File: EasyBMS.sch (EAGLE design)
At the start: 143 parts, among them Q10 BSS84LT1G, Q11 BSS84LT1G, Q12 BSS84LT1G, Q13 BSS84LT1G, Q2 BSS84LT1G, Q3 BSS84LT1G, Q4 BSS84LT1G, Q5 BSS84LT1G, Q6 BSS84LT1G, Q7 BSS84LT1G, Q8 BSS84LT1G, Q9 BSS84LT1G

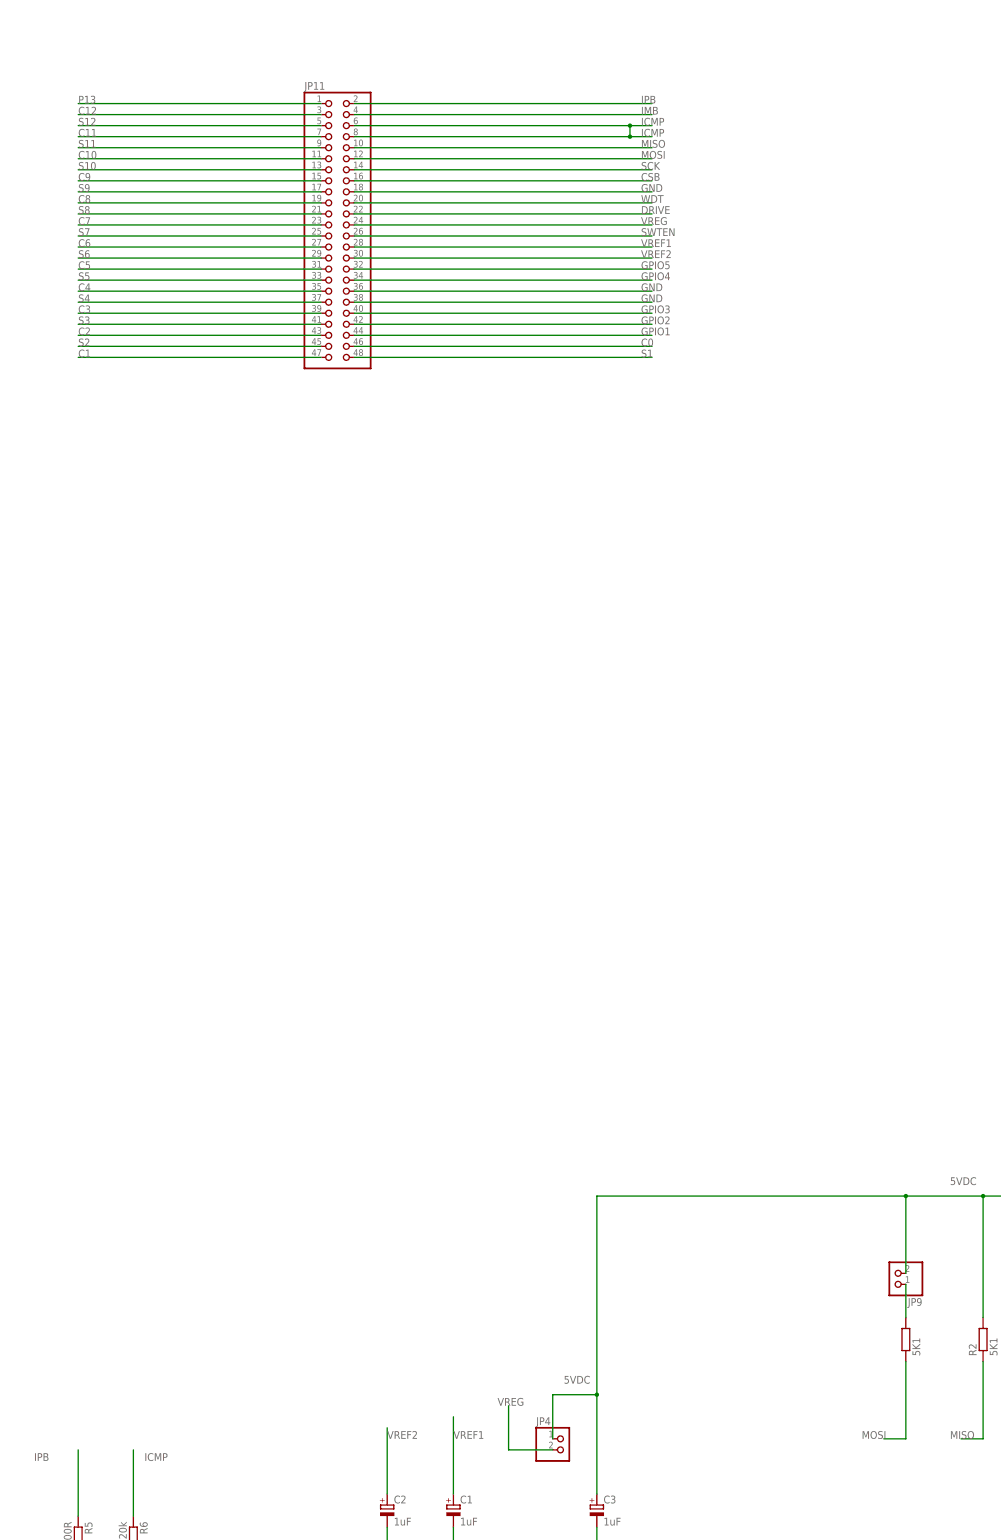
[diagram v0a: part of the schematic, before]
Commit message: new 2x20 header used
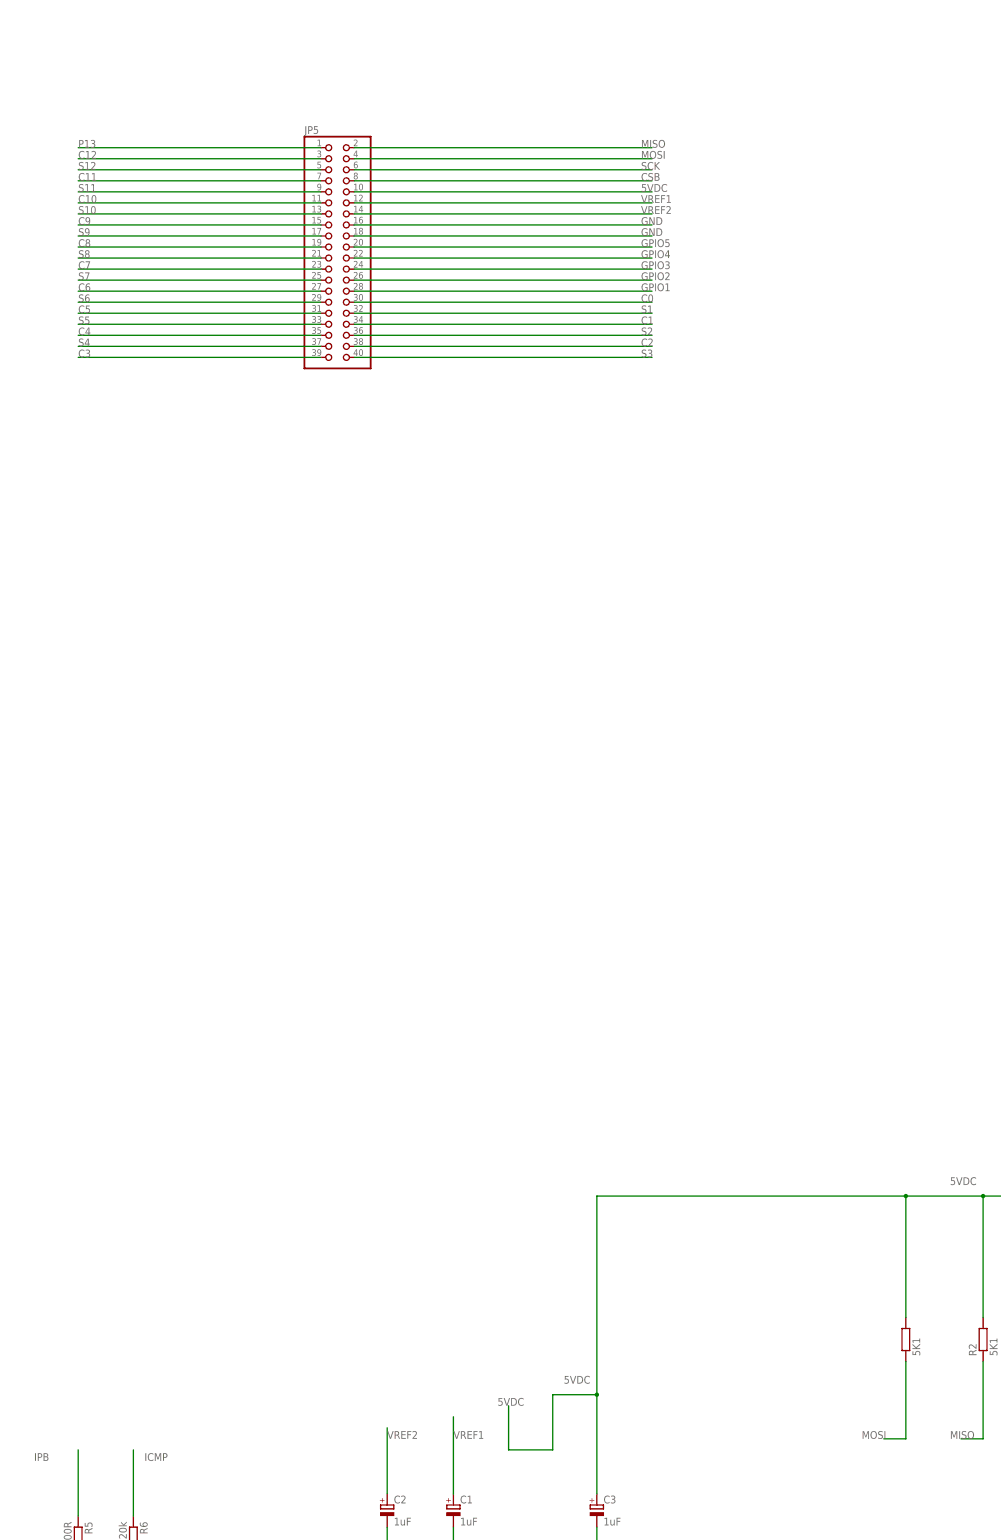
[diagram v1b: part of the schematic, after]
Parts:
- removed JP11: (no value), pinhead_own:PINHD-2X24
- removed JP4, JP9: (no value), pinhead_own:PINHD-1X2
- added JP5: (no value), pinhead:PINHD-2X20
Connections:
- removed net DRIVE: JP11.22
- removed net N$117: JP9.1, R1.2
- removed net SWTEN: JP11.26
- removed net VREG: JP11.24, JP4.2
- removed net WDT: JP11.20
- net 5VDC: now also JP5.10, R1.2; no longer JP4.1, JP9.2
- net C0: now also JP5.30; no longer JP11.46
- net C1: now also JP5.34; no longer JP11.47
- net C10: now also JP5.11; no longer JP11.11
- net C11: now also JP5.7; no longer JP11.7
- net C12: now also JP5.3; no longer JP11.3
- net C2: now also JP5.38; no longer JP11.43
- net C3: now also JP5.39; no longer JP11.39
- net C4: now also JP5.35; no longer JP11.35
- net C5: now also JP5.31; no longer JP11.31
- net C6: now also JP5.27; no longer JP11.27
- net C7: now also JP5.23; no longer JP11.23
- net C8: now also JP5.19; no longer JP11.19
- net C9: now also JP5.15; no longer JP11.15
- net CSB: now also JP5.8; no longer JP11.16
- net GND: now also JP5.16, JP5.18; no longer JP11.18, JP11.36, JP11.38
- net GPIO1: now also JP5.28; no longer JP11.44
- net GPIO2: now also JP5.26; no longer JP11.42
- net GPIO3: now also JP5.24; no longer JP11.40
- net GPIO4: now also JP5.22; no longer JP11.34
- net GPIO5: now also JP5.20; no longer JP11.32
- net ICMP: no longer JP11.6, JP11.8
- net IMB: no longer JP11.4
- net IPB: no longer JP11.2
- net MISO: now also JP5.2; no longer JP11.10
- net MOSI: now also JP5.4; no longer JP11.12
- net P13: now also JP5.1; no longer JP11.1
- net S1: now also JP5.32; no longer JP11.48
- net S10: now also JP5.13; no longer JP11.13
- net S11: now also JP5.9; no longer JP11.9
- net S12: now also JP5.5; no longer JP11.5
- net S2: now also JP5.36; no longer JP11.45
- net S3: now also JP5.40; no longer JP11.41
- net S4: now also JP5.37; no longer JP11.37
- net S5: now also JP5.33; no longer JP11.33
- net S6: now also JP5.29; no longer JP11.29
- net S7: now also JP5.25; no longer JP11.25
- net S8: now also JP5.21; no longer JP11.21
- net S9: now also JP5.17; no longer JP11.17
- net SCK: now also JP5.6; no longer JP11.14
- net VREF1: now also JP5.12; no longer JP11.28
- net VREF2: now also JP5.14; no longer JP11.30

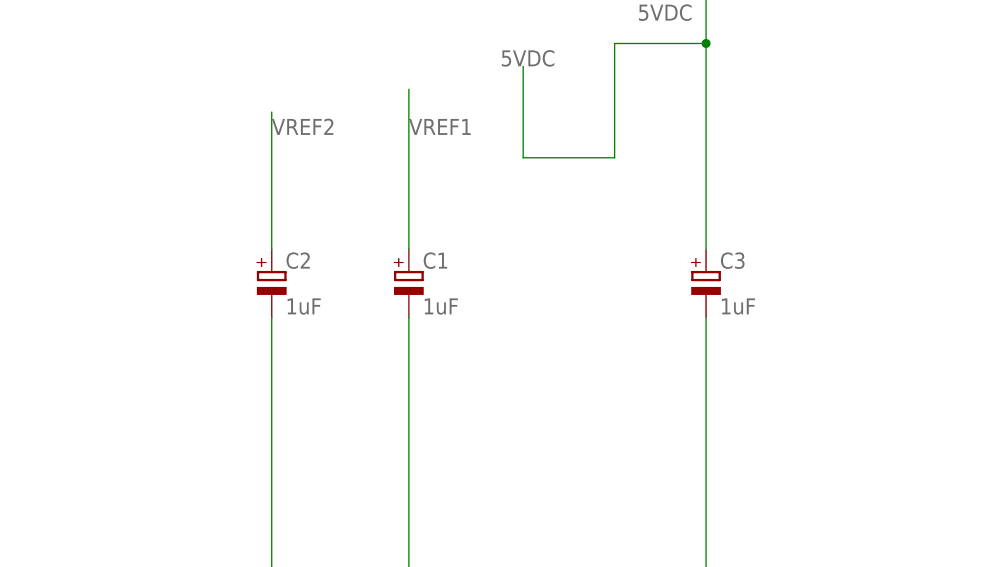
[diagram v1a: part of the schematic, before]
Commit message: positioning
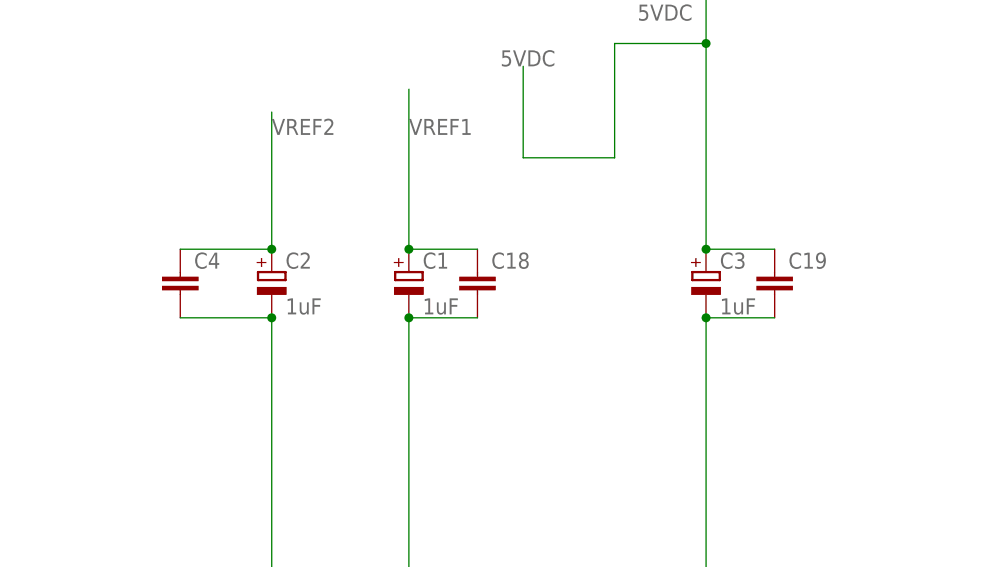
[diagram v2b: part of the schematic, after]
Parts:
- added C18, C19, C4: (no value), rcl:C-EUC1206
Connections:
- net 5VDC: now also C19.1
- net GND: now also C18.2, C19.2, C4.2
- net VREF1: now also C18.1
- net VREF2: now also C4.1
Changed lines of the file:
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@@
 <part name="R95" library="rcl" library_urn="urn:adsk.eagle:library:334" deviceset="R-EU_" device="R0402" package3d_urn="urn:adsk.eagle:package:23547/1" value="100R"/>
 <part name="JP5" library="pinhead" library_urn="urn:adsk.eagle:library:325" deviceset="PINHD-2X20" device="" package3d_urn="urn:adsk.eagle:package:22443/2"/>
+<part name="C4" library="rcl" library_urn="urn:adsk.eagle:library:334" deviceset="C-EU" device="C1206" package3d_urn="urn:adsk.eagle:package:23618/2"/>
+<part name="C18" library="rcl" library_urn="urn:adsk.eagle:library:334" deviceset="C-EU" device="C1206" package3d_urn="urn:adsk.eagle:package:23618/2"/>
+<part name="C19" library="rcl" library_urn="urn:adsk.eagle:library:334" deviceset="C-EU" device="C1206" package3d_urn="urn:adsk.eagle:package:23618/2"/>
 </parts>
 <sheets>
@@
 <attribute name="NAME" x="130.81" y="346.075" size="1.778" layer="95"/>
 <attribute name="VALUE" x="130.81" y="289.56" size="1.778" layer="96"/>
+</instance>
+<instance part="C4" gate="G$1" x="139.7" y="30.48" smashed="yes">
+<attribute name="NAME" x="141.224" y="30.861" size="1.778" layer="95"/>
+<attribute name="VALUE" x="141.224" y="25.781" size="1.778" layer="96"/>
+</instance>
+<instance part="C18" gate="G$1" x="172.72" y="30.48" smashed="yes">
+<attribute name="NAME" x="174.244" y="30.861" size="1.778" layer="95"/>
+<attribute name="VALUE" x="174.244" y="25.781" size="1.778" layer="96"/>
+</instance>
+<instance part="C19" gate="G$1" x="205.74" y="30.48" smashed="yes">
+<attribute name="NAME" x="207.264" y="30.861" size="1.778" layer="95"/>
+<attribute name="VALUE" x="207.264" y="25.781" size="1.778" layer="96"/>
 </instance>
 </instances>
@@
 <wire x1="187.96" y1="43.18" x2="177.8" y2="43.18" width="0.1524" layer="91"/>
 <pinref part="R1" gate="G$1" pin="2"/>
+<pinref part="C19" gate="G$1" pin="1"/>
+<wire x1="205.74" y1="33.02" x2="198.12" y2="33.02" width="0.1524" layer="91"/>
+<junction x="198.12" y="33.02"/>
 </segment>
 <segment>
@@
 <wire x1="91.44" y1="17.78" x2="91.44" y2="-22.86" width="0.1524" layer="91"/>
 <wire x1="91.44" y1="-22.86" x2="149.86" y2="-22.86" width="0.1524" layer="91"/>
+<pinref part="C4" gate="G$1" pin="2"/>
+<wire x1="139.7" y1="25.4" x2="149.86" y2="25.4" width="0.1524" layer="91"/>
+<junction x="149.86" y="25.4"/>
+<pinref part="C18" gate="G$1" pin="2"/>
+<wire x1="172.72" y1="25.4" x2="165.1" y2="25.4" width="0.1524" layer="91"/>
+<junction x="165.1" y="25.4"/>
+<pinref part="C19" gate="G$1" pin="2"/>
+<wire x1="205.74" y1="25.4" x2="198.12" y2="25.4" width="0.1524" layer="91"/>
+<junction x="198.12" y="25.4"/>
 </segment>
 <segment>
@@
 <wire x1="165.1" y1="50.8" x2="165.1" y2="33.02" width="0.1524" layer="91"/>
 <label x="165.1" y="45.72" size="1.778" layer="95"/>
+<pinref part="C18" gate="G$1" pin="1"/>
+<wire x1="165.1" y1="33.02" x2="172.72" y2="33.02" width="0.1524" layer="91"/>
+<junction x="165.1" y="33.02"/>
 </segment>
 <segment>
@@
 <wire x1="149.86" y1="48.26" x2="149.86" y2="33.02" width="0.1524" layer="91"/>
 <label x="149.86" y="45.72" size="1.778" layer="95"/>
-</segment>
-<segment>
+<pinref part="C4" gate="G$1" pin="1"/>
+<wire x1="149.86" y1="33.02" x2="139.7" y2="33.02" width="0.1524" layer="91"/>
+<junction x="149.86" y="33.02"/>
+</segment>
+<segment>
